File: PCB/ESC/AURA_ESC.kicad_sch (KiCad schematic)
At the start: 70 parts, among them J1 Conn_01x03_Pin, J2 Conn_01x04_Pin, J3 Conn_01x01_Pin, J4 Conn_01x01_Pin, J5 Conn_01x01_Pin, J6 Conn_01x01_Pin, J7 Conn_01x01_Pin, U1 STM32F051K8U6, U10 SQJ138ELP-T1_GE3, U2 INA199A1DCKR, U3 AOZ1282CI, U4 AMS1117-3.3, U5 SQJ138ELP-T1_GE3, U6 SQJ138ELP-T1_GE3, U7 SQJ138ELP-T1_GE3, U8 SQJ138ELP-T1_GE3, U9 SQJ138ELP-T1_GE3

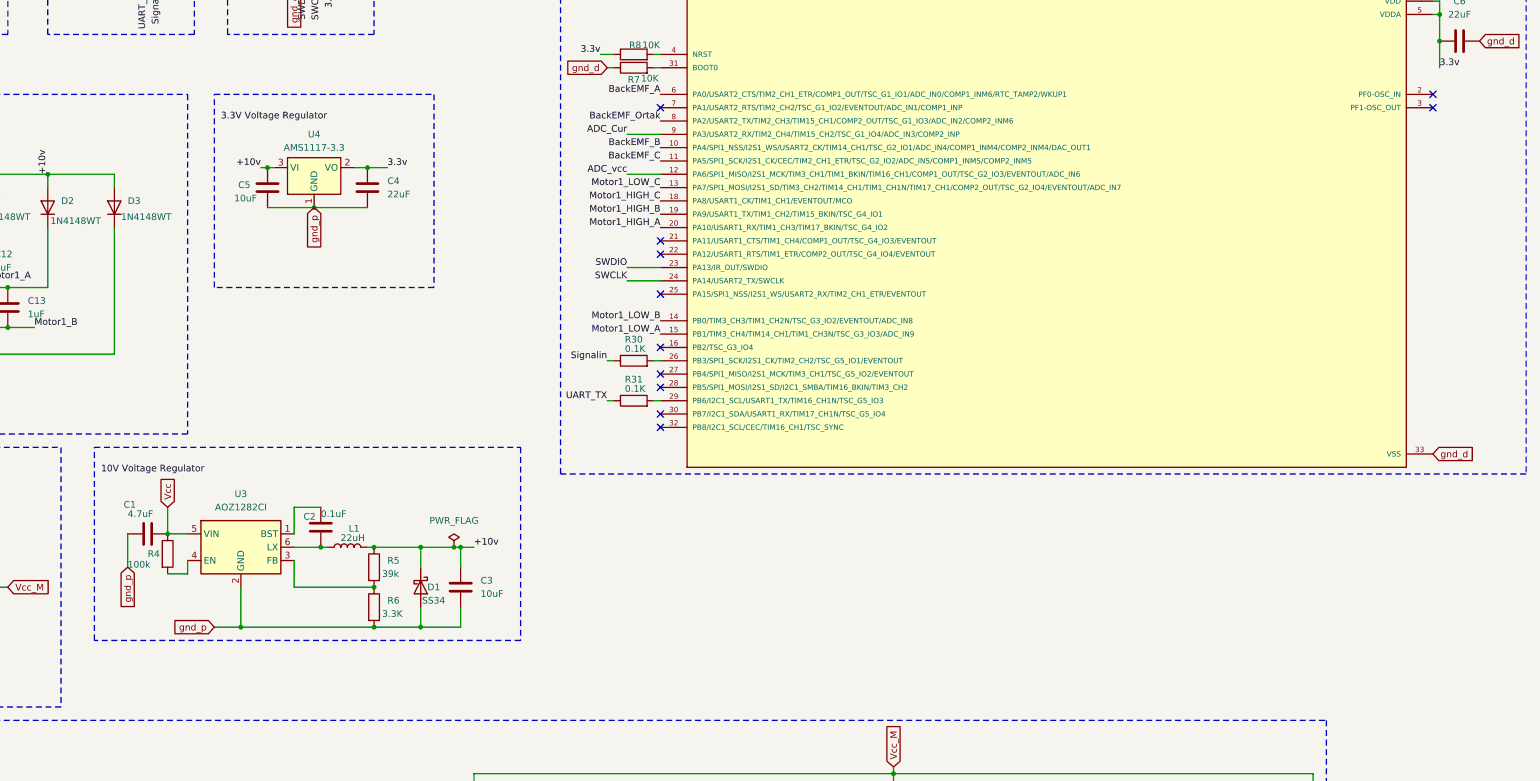
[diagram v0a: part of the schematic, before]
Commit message: Add files via upload
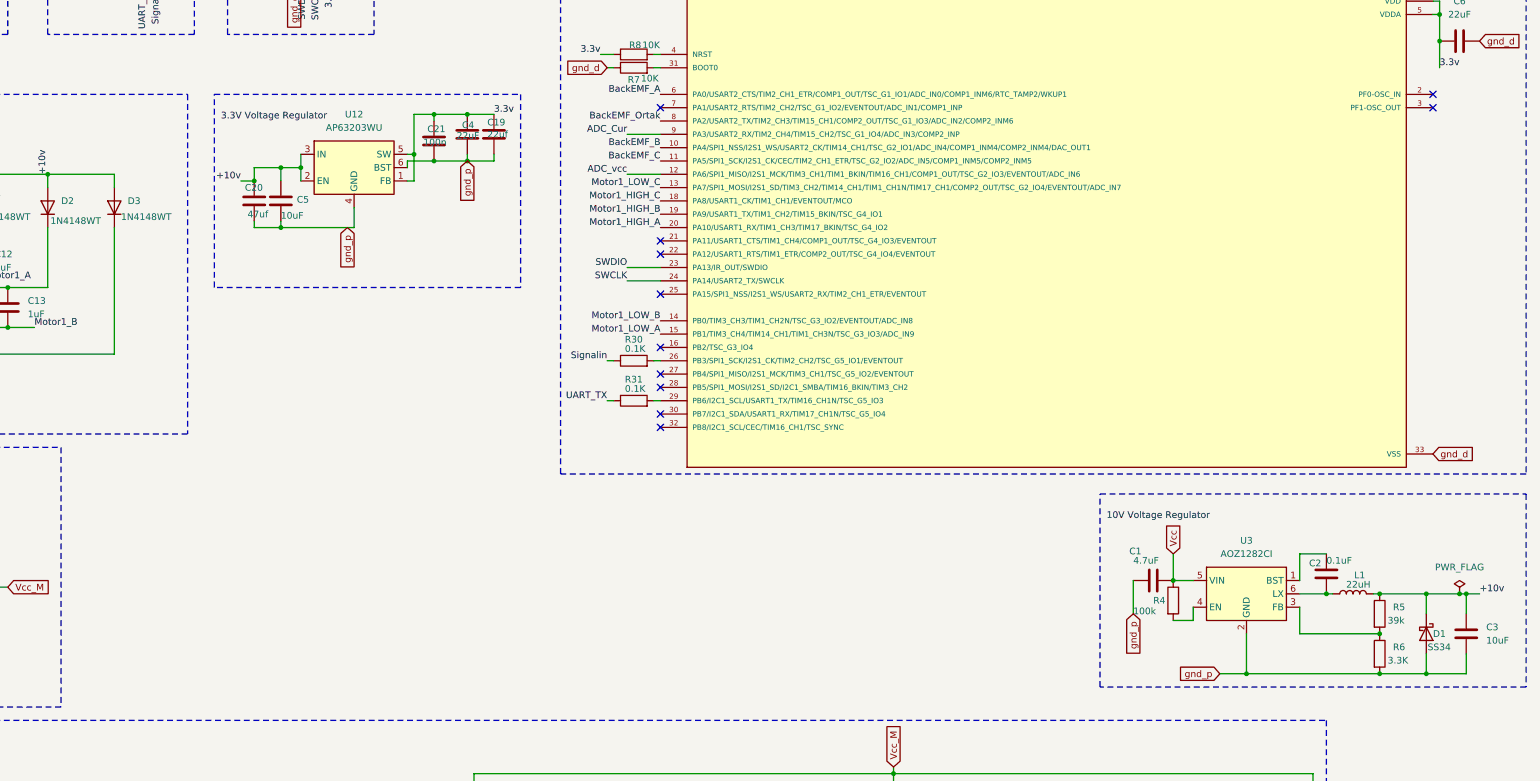
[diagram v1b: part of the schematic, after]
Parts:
- removed U4: AMS1117-3.3, Package_TO_SOT_SMD:SOT-223-3_TabPin2, symbol Regulator_Linear:AMS1117-3.3
- added C19: 22uf, Capacitor_SMD:C_0201_0603Metric, symbol Device:C
- added C20: 47uf, Capacitor_SMD:C_0201_0603Metric, symbol Device:C
- added C21: 100n, Capacitor_SMD:C_0201_0603Metric, symbol Device:C
- added U12: AP63203WU, Package_TO_SOT_SMD:TSOT-23-6, symbol Regulator_Switching:AP63203WU
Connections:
- net +10v: now also C20.1, U12.2 (EN), U12.3 (IN)
- net VDD: now also C19.1, C21.1, U12.1 (FB), U12.5 (SW)
- net gnd_p: now also C19.2, C20.2, C21.2, U12.4 (GND), U12.6 (BST)
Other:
- moved on the sheet: C1, C2, C3, C4, C5, D1, L1, R4, R5, R6, U3
